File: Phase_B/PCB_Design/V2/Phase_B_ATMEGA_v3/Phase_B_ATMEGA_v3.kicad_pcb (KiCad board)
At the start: 2 copper layers, 103.5 x 103.5 mm, 53 parts, among them J1 AVR-ISP-6, J2 USB_B_Mini, J3 ESP_Conn, U1 CA56-12EWA, U2 74HC595, U3 ATmega32U4-A, U4 USBLC6-2SC6, U5 LP2985-3.3, Y1 16MHz

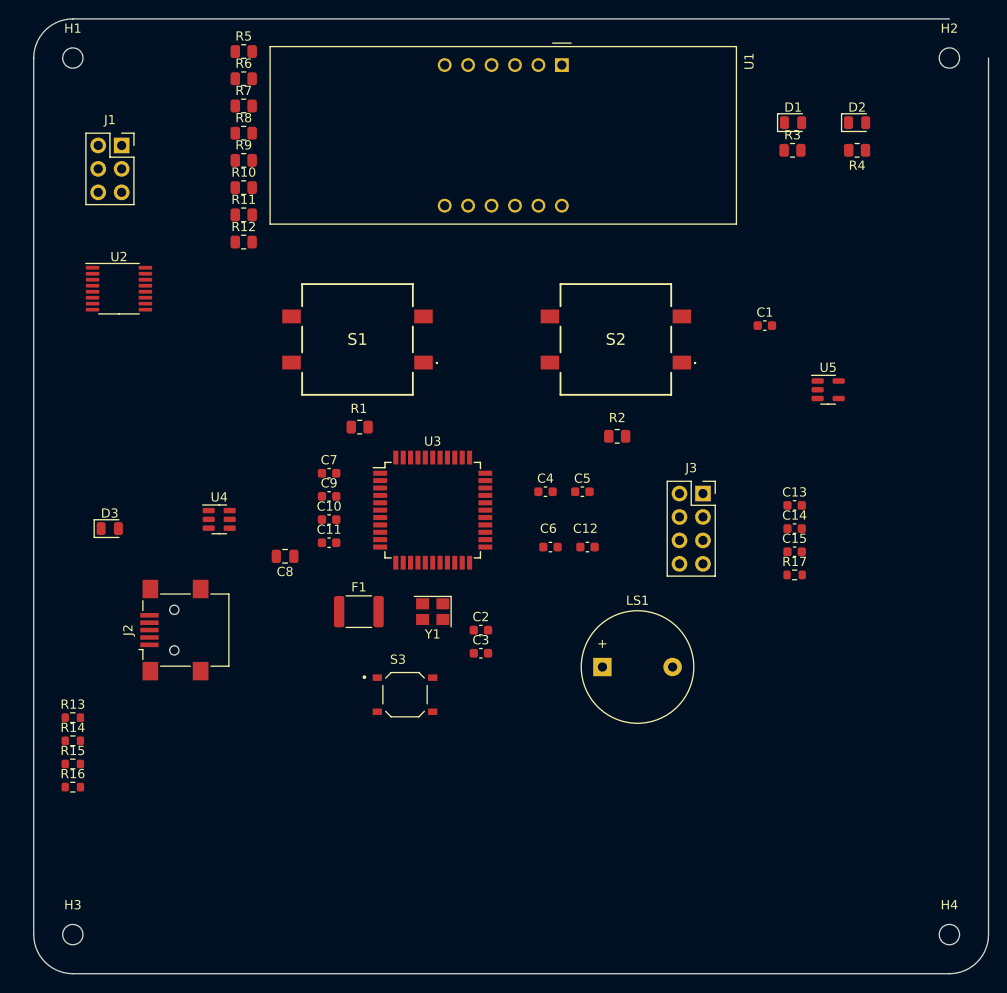
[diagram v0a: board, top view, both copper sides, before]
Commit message: Placement Tinkering
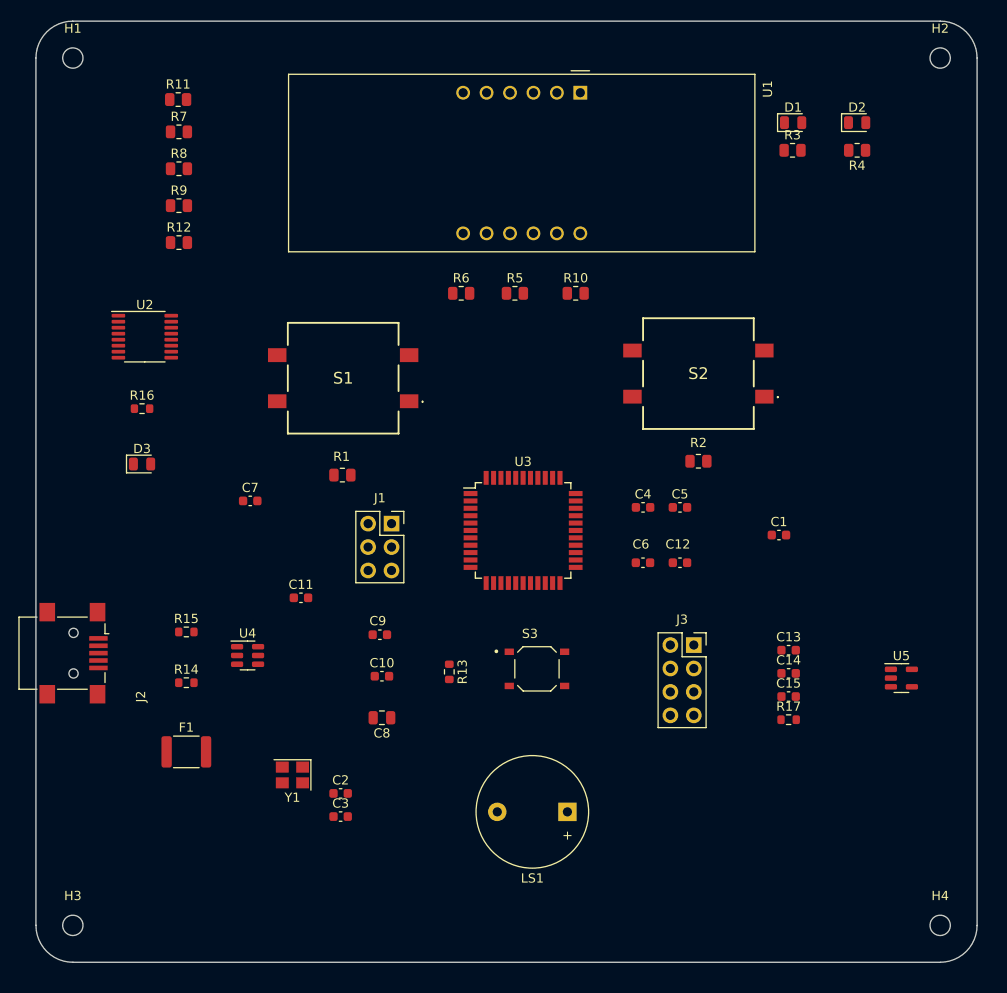
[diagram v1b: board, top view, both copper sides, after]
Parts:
- moved J1 50.4 mm to (94.5, 130.5)
- moved R16 41.7 mm to (67.5, 118.0)
- moved R13 41.1 mm to (100.8, 146.5), turned to -90 degrees
- moved R5 39.4 mm to (107.9, 105.5)
- moved R10 37.8 mm to (114.5, 105.5)
- moved R6 33.1 mm to (102.1, 105.5)
- moved U5 32.2 mm to (149.8, 147.2)
- moved F1 24.1 mm to (72.3, 155.2)
- moved C3 23.3 mm to (89.0, 162.2)
- moved Y1 23.3 mm to (83.8, 157.7)
- moved C2 23.3 mm to (89.0, 159.7)
- moved C1 22.8 mm to (136.5, 131.7)
- moved C8 20.4 mm to (93.5, 151.5)
- moved R15 18.9 mm to (72.3, 142.2)
- moved C10 17.9 mm to (93.5, 147.0)
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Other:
- board size 103.5 x 103.5 mm -> 102 x 102 mm
